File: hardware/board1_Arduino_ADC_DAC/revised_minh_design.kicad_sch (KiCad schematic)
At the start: 36 parts, among them J1 Conn_01x03_Male, J2 Conn_02x08_Odd_Even, J3 Conn_02x08_Odd_Even, J4 Conn_02x08_Odd_Even, J5 Conn_01x02_Male, U1 ESP32-DevKit-C, U2 LM7805_TO220, U3 MCP1754S-3302xCB, U4 MCP1825S-3.3V, U5 MCP1501-33xSN, U6 MCP3464R, U7 MCP3464R, U8 DAC8568IAPW, X1 ECS-2520MVLC-049-BN-TR

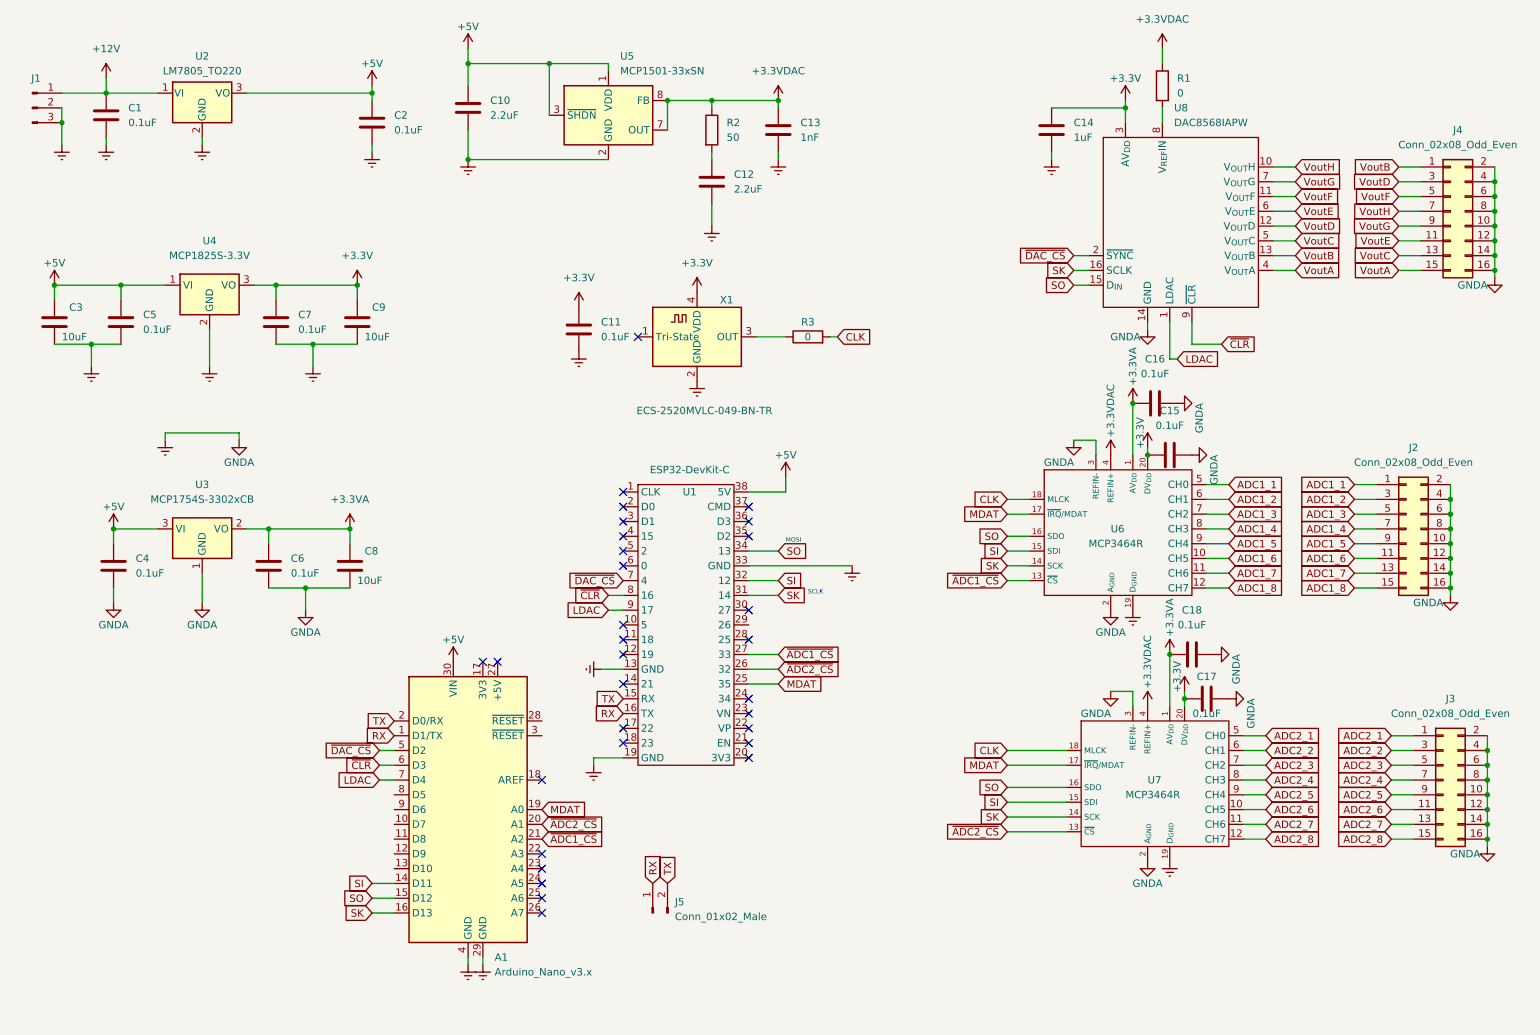
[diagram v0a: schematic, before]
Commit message: cleanup
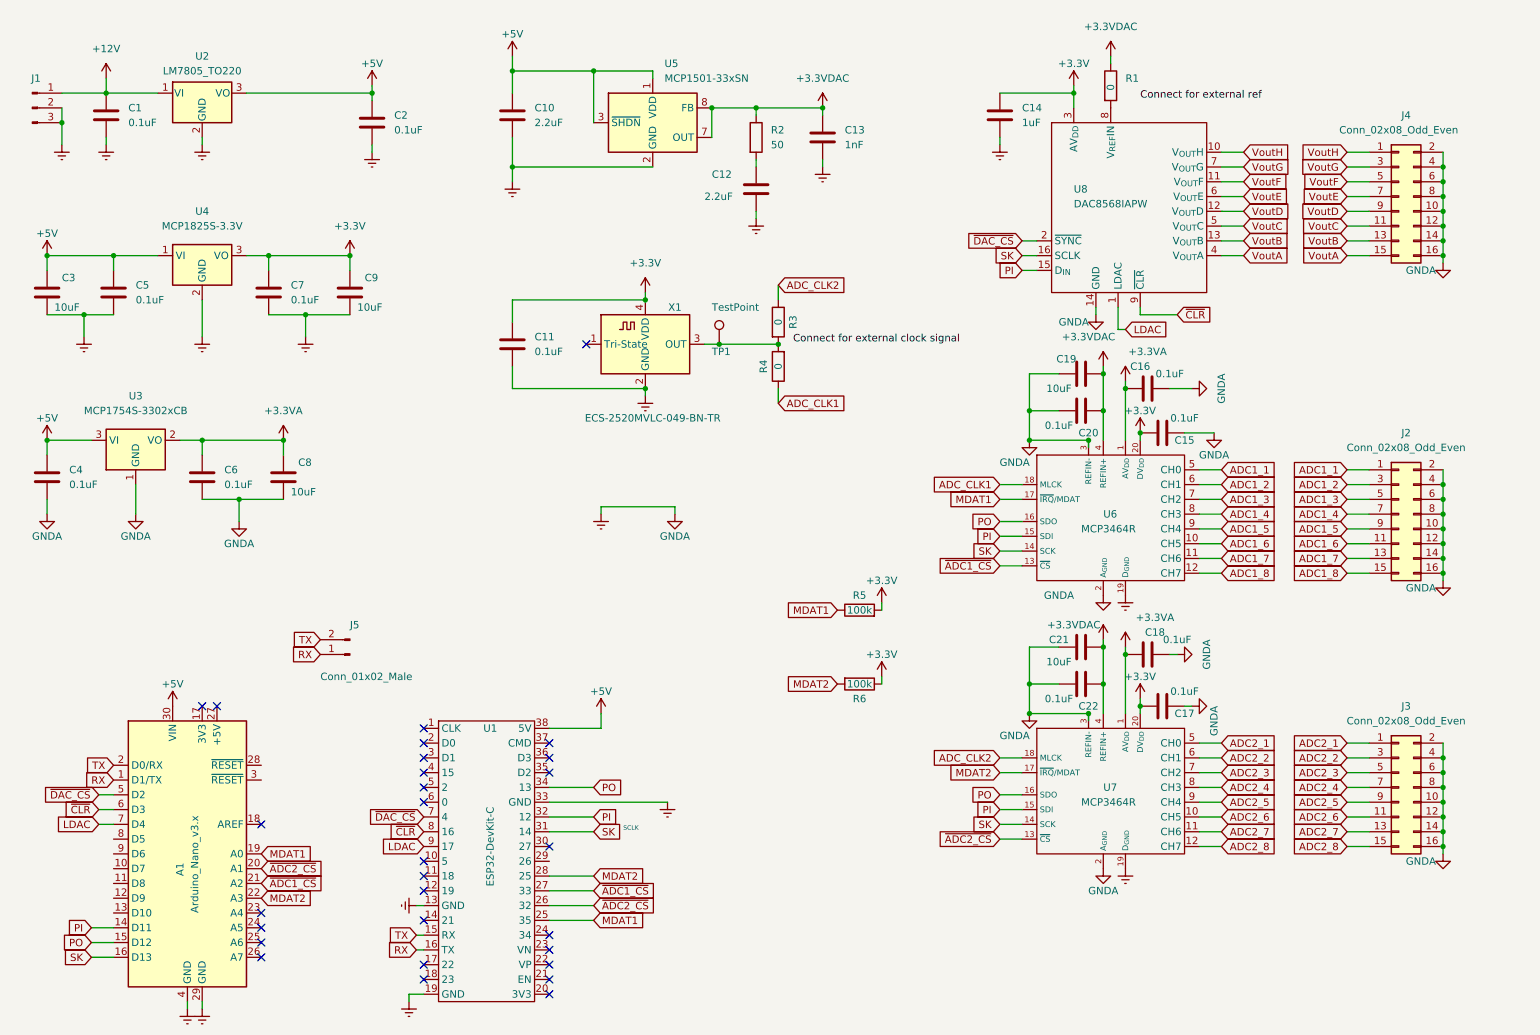
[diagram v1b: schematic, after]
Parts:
- added C19, C21: 10uF, Capacitor_SMD:C_0805_2012Metric_Pad1.18x1.45mm_HandSolder, symbol Device:C
- added C20, C22: 0.1uF, Capacitor_SMD:C_0805_2012Metric_Pad1.18x1.45mm_HandSolder, symbol Device:C
- added R4: 0, Resistor_SMD:R_0805_2012Metric_Pad1.20x1.40mm_HandSolder, symbol Device:R
- added R5, R6: 100k, Resistor_SMD:R_0805_2012Metric_Pad1.20x1.40mm_HandSolder, symbol Device:R
- added TP1: TestPoint, Connector_PinHeader_2.54mm:PinHeader_1x01_P2.54mm_Vertical, symbol Connector:TestPoint
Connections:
- net +3.3VDAC: now also C19.1, C20.1, C21.1, C22.1
- net +3V3: now also R5.2, R6.1
- net Earth: now also C19.2, C20.2, C21.2, C22.2
- net VoutB: now also J4.13 (Pin_13); no longer J4.1 (Pin_1)
- net VoutC: now also J4.11 (Pin_11); no longer J4.13 (Pin_13)
- net VoutD: now also J4.9 (Pin_9); no longer J4.3 (Pin_3)
- net VoutE: now also J4.7 (Pin_7); no longer J4.11 (Pin_11)
- net VoutG: now also J4.3 (Pin_3); no longer J4.9 (Pin_9)
- net VoutH: now also J4.1 (Pin_1); no longer J4.7 (Pin_7)
- net at X1.3 (OUT): now also R3.2, R4.2, TP1.1; no longer R3.1
- net MDAT2: now reaches A1.22 (A3)
- net MDAT2: now also U1.28 (25), U7.17 (~{IRQ}/MDAT), R6.2
- removed net CLK: R3.2, U6.18 (MLCK), U7.18 (MLCK)
- net MDAT renamed MDAT1
- net MDAT1: now also R5.1; no longer U7.17 (~{IRQ}/MDAT)
- net SI renamed PI
- net PI: now also U8.15 (D_{IN})
- net SO renamed PO
- net PO: no longer U8.15 (D_{IN})
- new net ADC_CLK1: R4.1, U6.18 (MLCK)
- new net ADC_CLK2: R3.1, U7.18 (MLCK)
- no-connect marks 31 -> 29
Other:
- note removed: "MOSI"
- title: (none) -> S.H.V.R.I.M.P.S.    16 channels data acquisition device
- moved on the sheet: A1, C10, C11, C12, C13, C14, C15, C16, C17, C18, C3, C4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
